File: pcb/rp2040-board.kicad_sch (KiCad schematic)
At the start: 32 parts, among them SW1 USB Boot, SW2 Reset, U1 RP2040, U2 W25Q128JVS, U3 SP485EEN-L/TR, Y1 12MHz

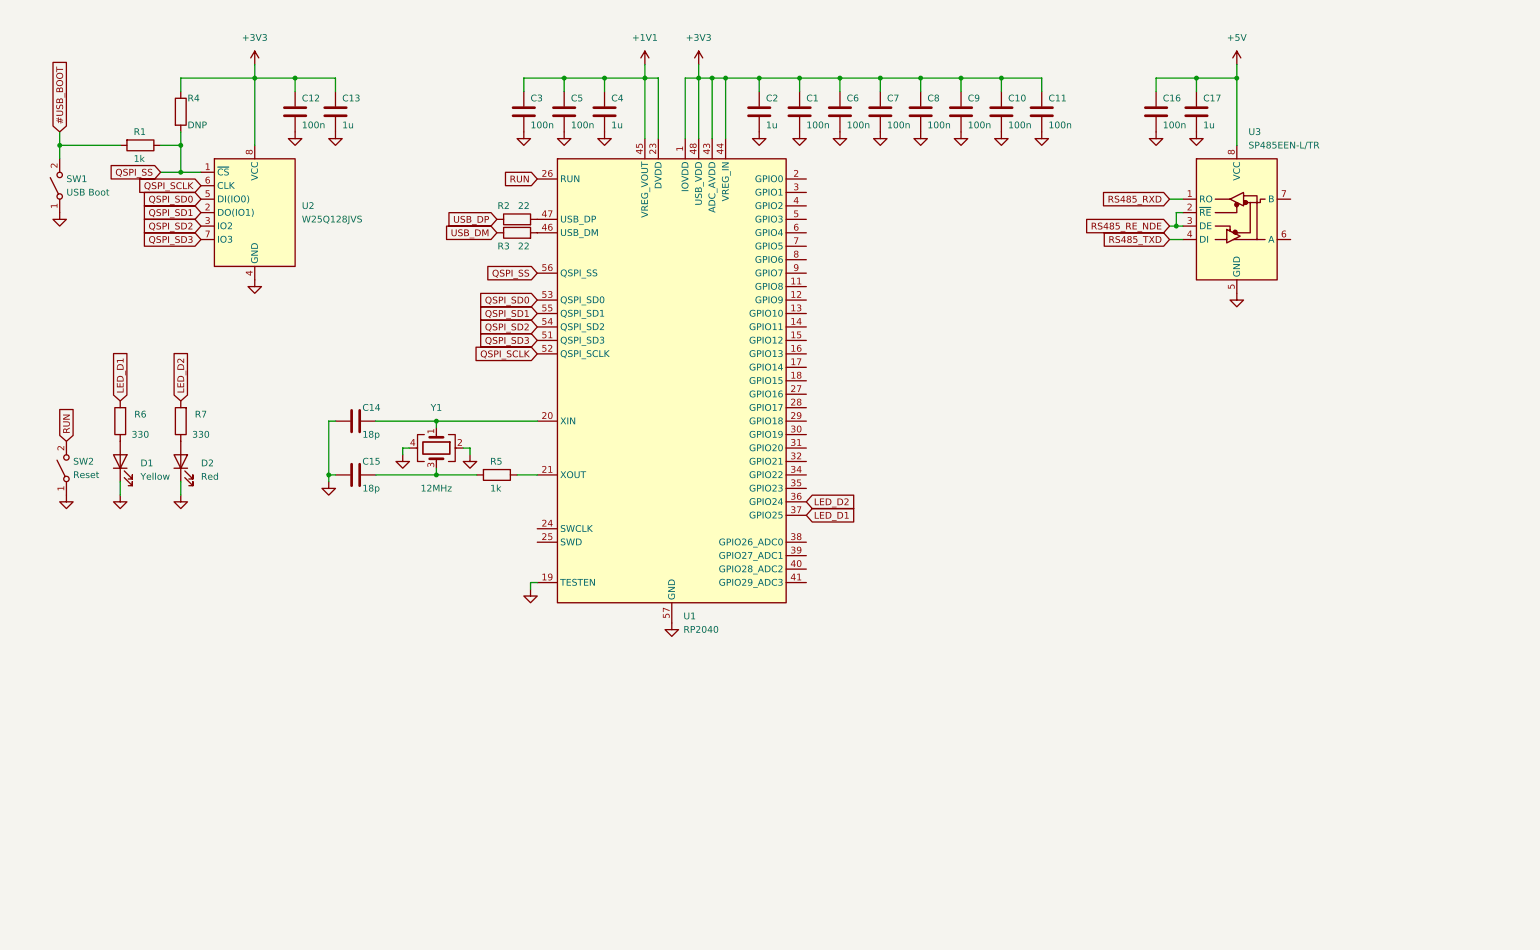
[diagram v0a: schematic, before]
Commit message: schematic wip
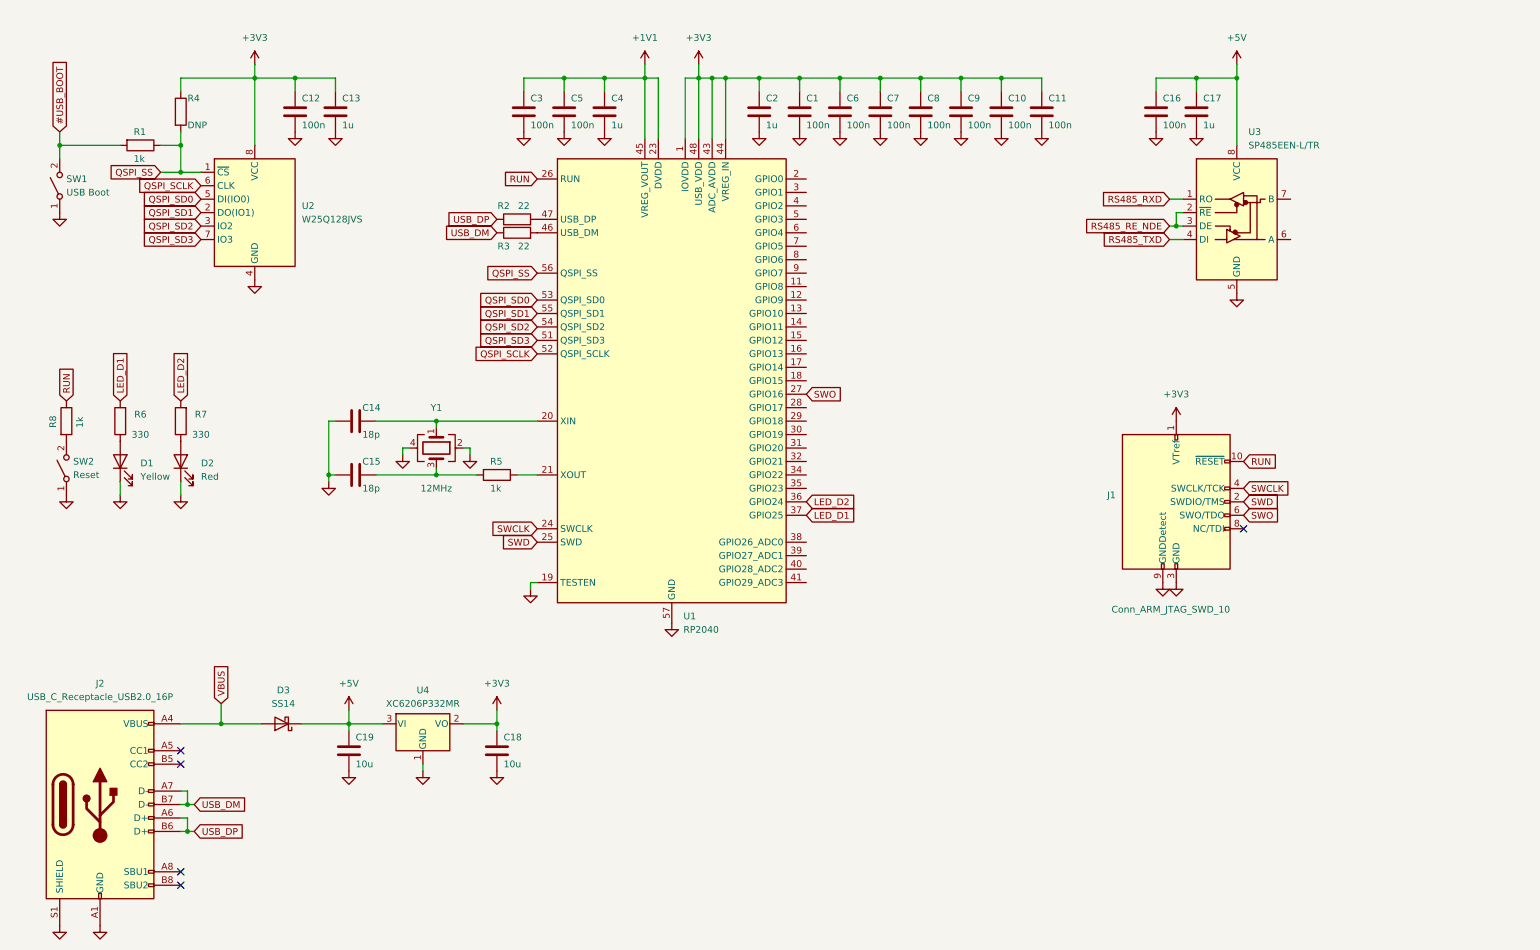
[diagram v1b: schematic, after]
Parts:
- added C18, C19: 10u, Capacitor_SMD:C_0603_1608Metric, symbol Device:C
- added D3: SS14, Diode_SMD:D_SMA, symbol Device:D_Schottky
- added J1: Conn_ARM_JTAG_SWD_10, symbol Connector:Conn_ARM_JTAG_SWD_10
- added J2: USB_C_Receptacle_USB2.0_16P, Connector_USB:USB_C_Receptacle_G-Switch_GT-USB-7010ASV, symbol Connector:USB_C_Receptacle_USB2.0_16P
- added R8: 1k, Resistor_SMD:R_0402_1005Metric, symbol Device:R
- added U4: XC6206P332MR, Package_TO_SOT_SMD:SOT-23-3, symbol Regulator_Linear:XC6206PxxxMR
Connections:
- net +3V3: now also C18.1, J1.1 (VTref), U4.2 (VO)
- net +5V: now also C19.1, D3.1 (K), U4.3 (VI)
- net GND: now also C18.2, C19.2, J1.3 (GND), J1.5 (GND), J1.9 (GNDDetect), J2.A1 (GND), J2.A12 (GND), J2.B1 (GND), J2.B12 (GND), J2.S1 (SHIELD), U4.1 (GND)
- net RUN: now also J1.10 (~{RESET}), R8.1; no longer SW2.2 (B)
- net USB_DM: now also J2.A7 (D-), J2.B7 (D-)
- net USB_DP: now also J2.A6 (D+), J2.B6 (D+)
- net SWCLK: now reaches U1.24 (SWCLK)
- net SWCLK: now also J1.4 (SWCLK/TCK)
- net SWD: now reaches U1.25 (SWD)
- net SWD: now also J1.2 (SWDIO/TMS)
- net SWO: now reaches U1.27 (GPIO16)
- net SWO: now also J1.6 (SWO/TDO)
- new net: R8.2, SW2.2 (B)
- new net VBUS: D3.2 (A), J2.A4 (VBUS), J2.A9 (VBUS), J2.B4 (VBUS), J2.B9 (VBUS)
- no-connect marks 0 -> 5

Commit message: schematic wip
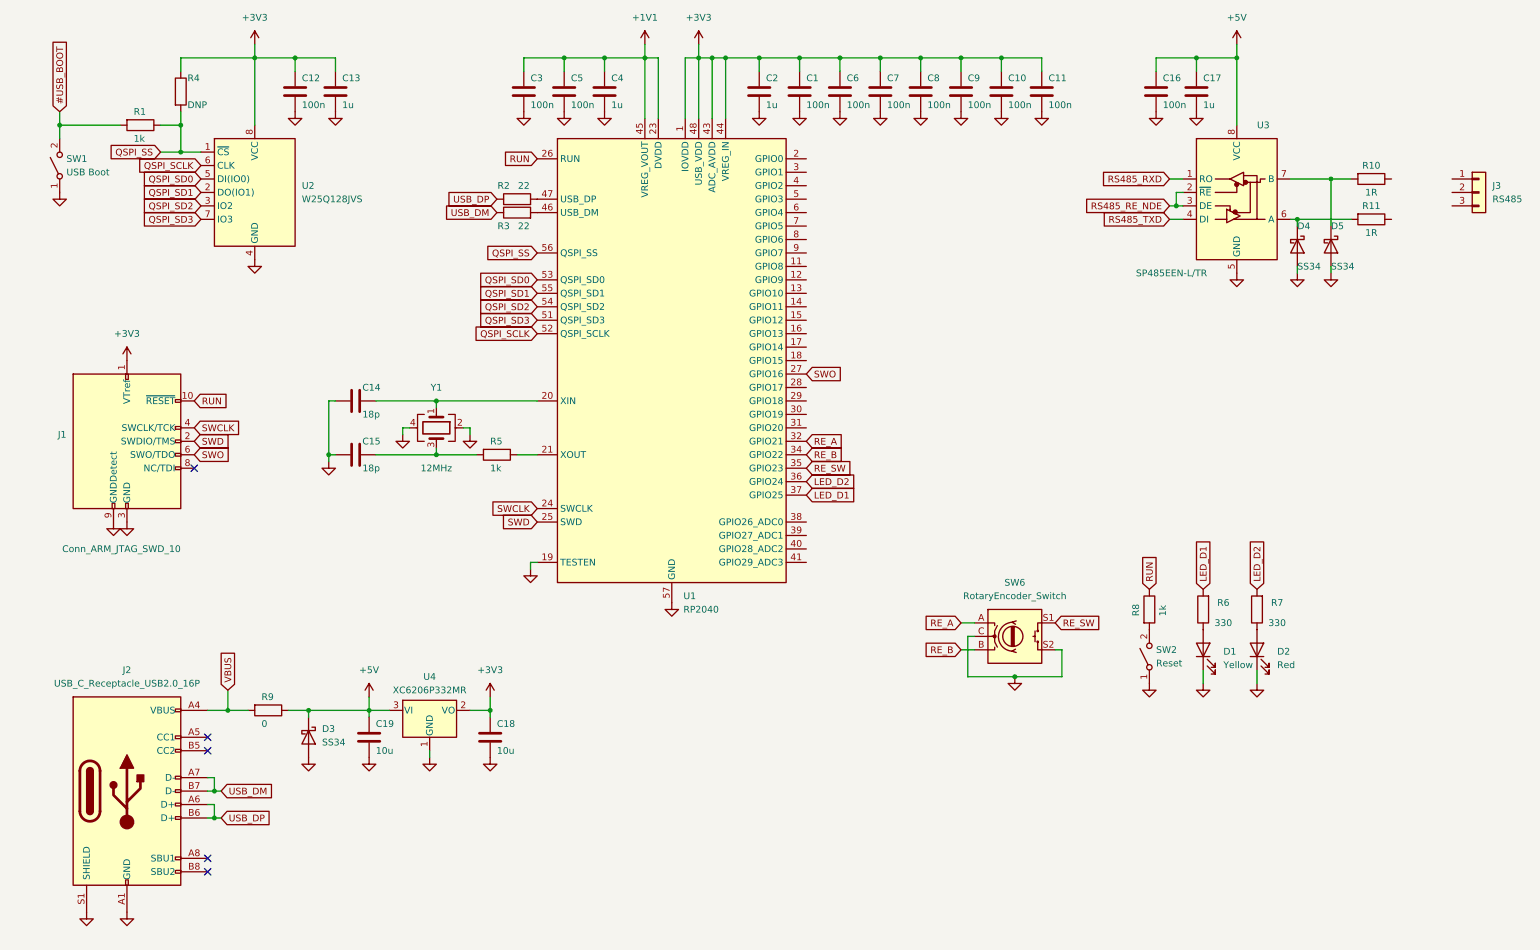
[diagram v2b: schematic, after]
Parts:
- added D4, D5: SS34, Diode_SMD:D_SMA, symbol Device:D_Schottky
- added J3: RS485, Connector_PinHeader_2.54mm:PinHeader_1x03_P2.54mm_Vertical, symbol Connector_Generic:Conn_01x03
- added R10, R11: 1R, Resistor_SMD:R_0603_1608Metric, symbol Device:R
- added R9: 0, Resistor_SMD:R_0402_1005Metric, symbol Device:R
- added SW6: RotaryEncoder_Switch, symbol Device:RotaryEncoder_Switch
- D3: value SS14 -> SS34; LCSC Part C2480 -> C8678
- J1: footprint (none) -> Connector_PinHeader_1.27mm:PinHeader_2x05_P1.27mm_Vertical_SMD
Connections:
- net +5V: now also R9.1
- net GND: now also D3.2 (A), D4.2 (A), D5.2 (A), SW6.C, SW6.S2
- net VBUS: now also R9.2; no longer D3.2 (A)
- net at U3.6 (A): now also D4.1 (K), R11.2
- net at U3.7 (B): now also D5.1 (K), R10.2
- net RE_A: now reaches U1.32 (GPIO21)
- net RE_A: now also SW6.A
- net RE_B: now reaches U1.34 (GPIO22)
- net RE_B: now also SW6.B
- net RE_SW: now reaches U1.35 (GPIO23)
- net RE_SW: now also SW6.S1
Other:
- moved on the sheet: C1, C10, C11, C12, C13, C14, C15, C16, C17, C18, C19, C2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

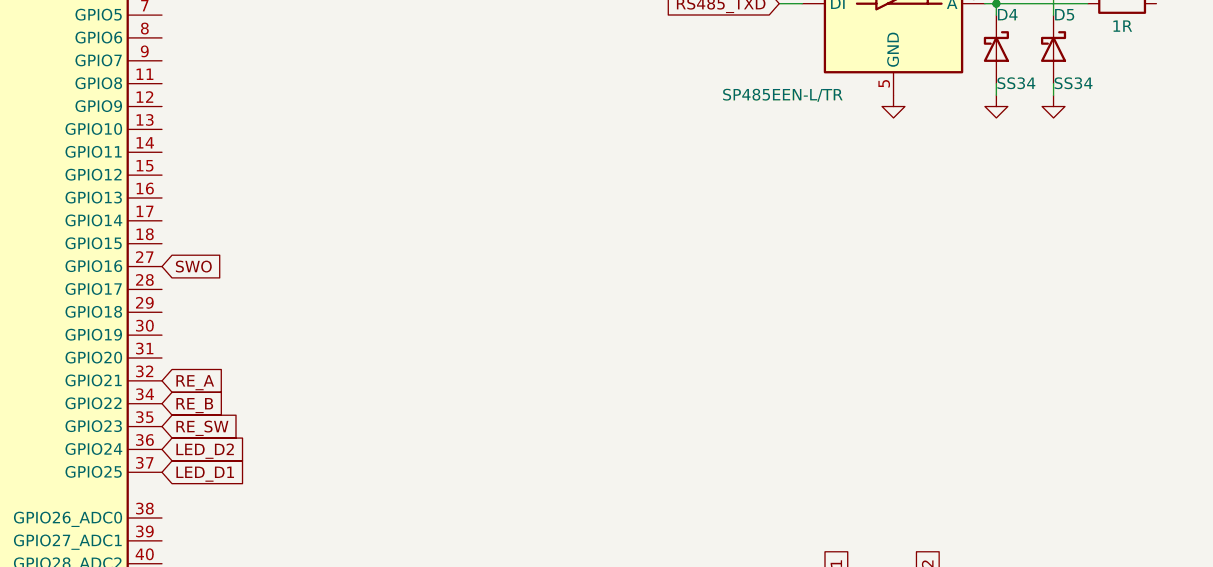
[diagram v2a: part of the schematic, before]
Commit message: schematic wip
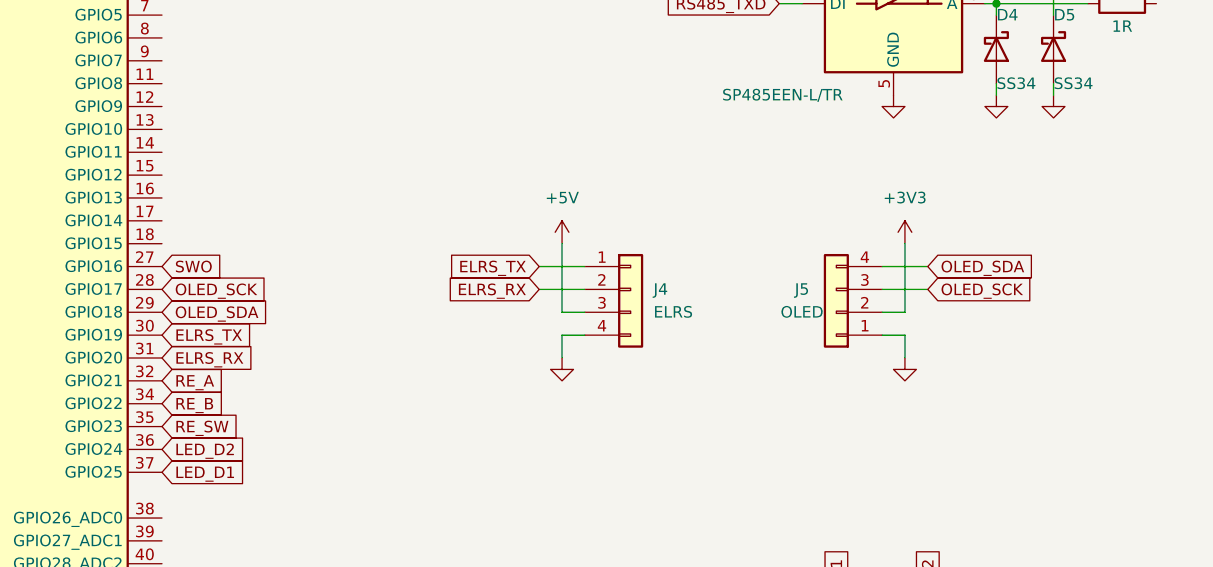
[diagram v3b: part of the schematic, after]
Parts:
- added J4: ELRS, Connector_PinHeader_2.54mm:PinHeader_1x04_P2.54mm_Vertical, symbol Connector_Generic:Conn_01x04
- added J5: OLED, Connector_PinHeader_2.54mm:PinHeader_1x04_P2.54mm_Vertical, symbol Connector_Generic:Conn_01x04
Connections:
- net +3V3: now also J5.2 (Pin_2)
- net +5V: now also J4.3 (Pin_3)
- net GND: now also J4.4 (Pin_4), J5.1 (Pin_1)
- net OLED_SCK: now reaches U1.28 (GPIO17)
- net OLED_SCK: now also J5.3 (Pin_3)
- net OLED_SDA: now reaches U1.29 (GPIO18)
- net OLED_SDA: now also J5.4 (Pin_4)
- net ELRS_TX: now reaches U1.30 (GPIO19)
- net ELRS_TX: now also J4.1 (Pin_1)
- net ELRS_RX: now reaches U1.31 (GPIO20)
- net ELRS_RX: now also J4.2 (Pin_2)
